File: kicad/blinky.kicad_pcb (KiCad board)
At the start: 2 copper layers, 40 x 39.9 mm, 17 parts, among them J2 Val**, Q1 MMBT2222, Q2 MMBT2222, Q3 MMBT2222, Q4 MMBT2222

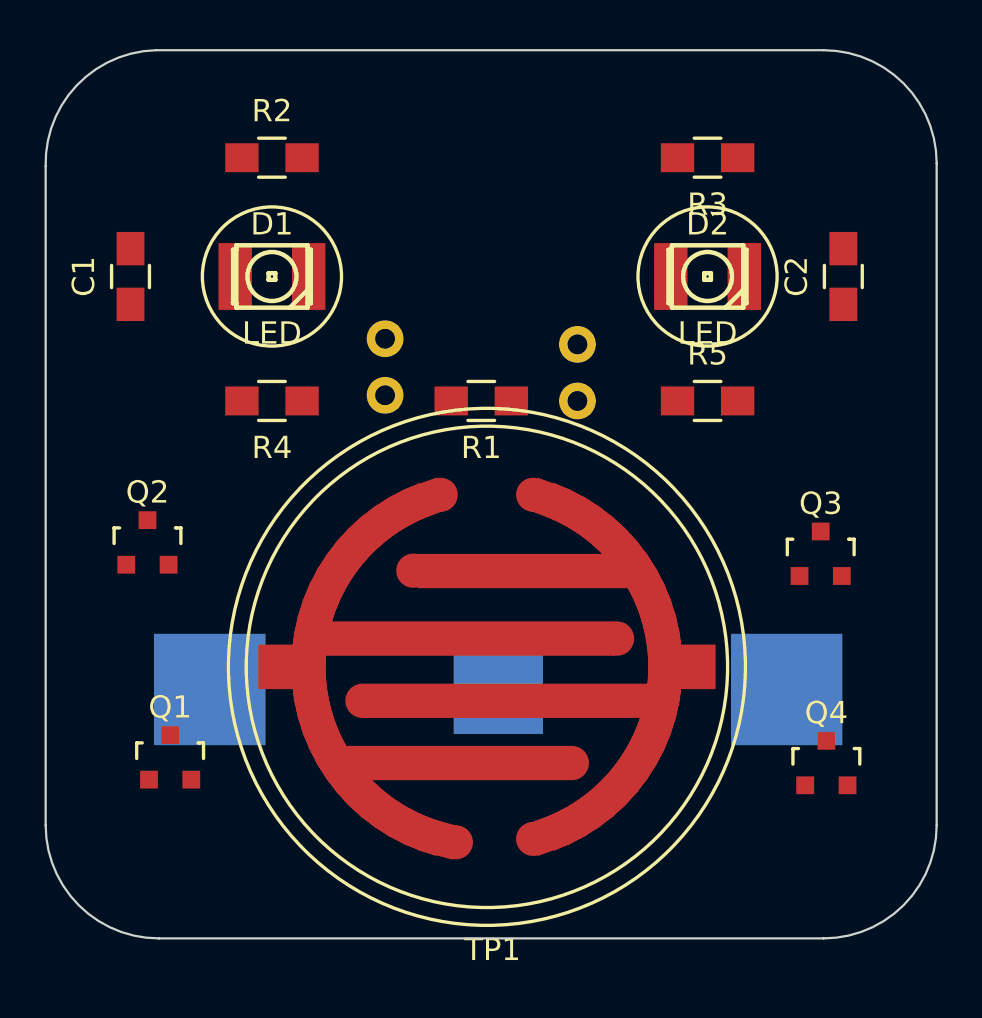
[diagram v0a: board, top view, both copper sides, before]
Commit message: routing done
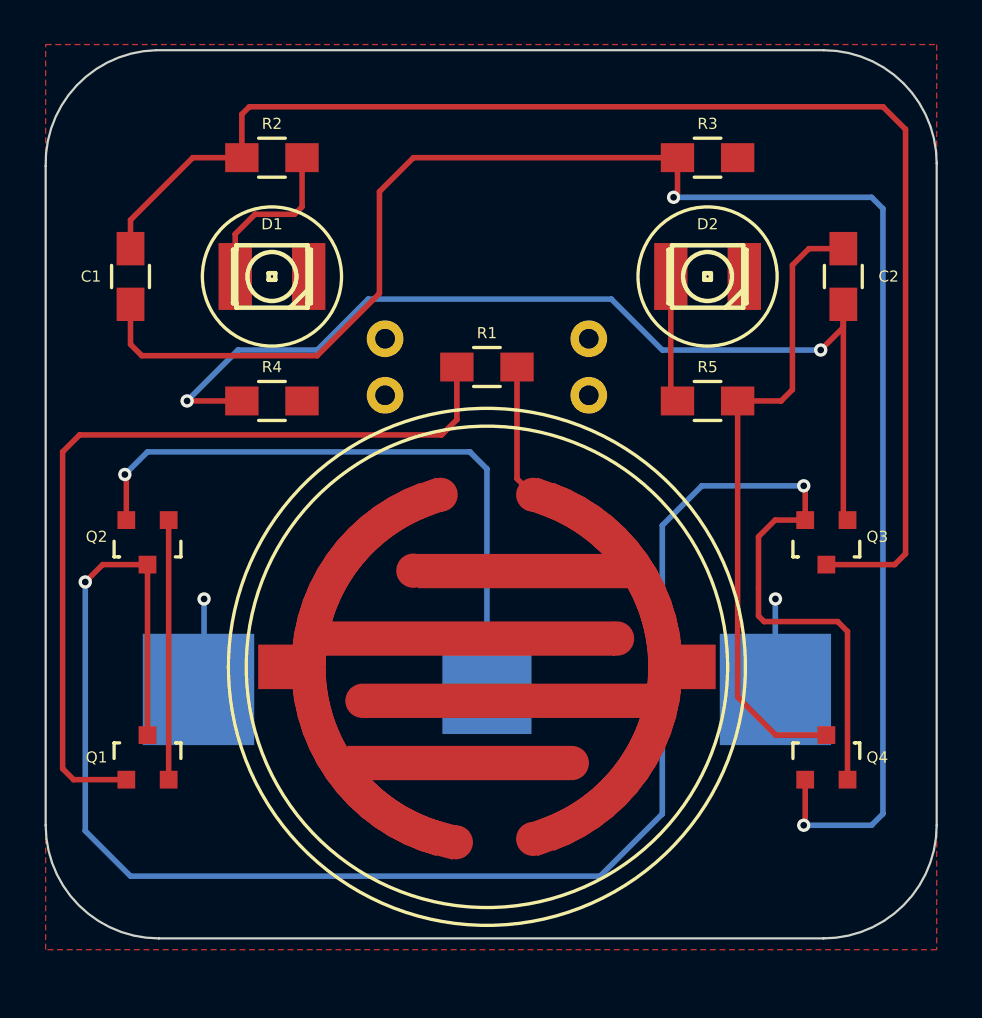
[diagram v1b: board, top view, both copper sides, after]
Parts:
- Q1, Q2, Q3, Q4: footprint Housings_SOT-23_SOT-143_TSOT-6:SOT-23 -> bb:SOT-23
- moved R1 1.55 mm to (148.1, 105.9)
- moved Q1 1.02 mm to (132.8, 123.4)
- moved J2 0.57 mm to (152.7, 105.9)
- moved Q3 0.57 mm to (163.3, 113.8), turned to 180 degrees
- moved BT1 0.51 mm to (148.1, 120.4)
- moved Q4 0.25 mm to (163.3, 123.4)
- turned C2 to 270 degrees
- turned Q2 to 180 degrees
- turned R2 to 180 degrees
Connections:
- net Net-(BT1-Pad1) renamed VCC
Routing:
- net Net-(Q1-Pad1): track 0.00 -> 88.4 mm, vias 0 -> 2
- net Net-(C1-Pad1): track 0.00 -> 77.4 mm, vias 0 -> 2
- net Net-(C1-Pad2): track 0.00 -> 62.6 mm
- net Net-(C2-Pad2): track 0.00 -> 46.0 mm, vias 0 -> 2
- net Net-(Q1-Pad2): track 0.00 -> 38.0 mm
- net GND: track 0.00 -> 29.0 mm, vias 0 -> 1
- net Net-(C2-Pad1): track 0.00 -> 28.8 mm
- net Net-(Q1-Pad3): track 0.00 -> 11.7 mm
- net VCC: track 0.00 -> 8.13 mm, vias 0 -> 2
- net Net-(D1-Pad1): track 0.00 -> 7.62 mm
- net Net-(R1-Pad1): track 0.00 -> 6.03 mm
- net Net-(D2-Pad1): track 0.00 -> 5.71 mm
- added copper zone on F.Cu, net VCC
